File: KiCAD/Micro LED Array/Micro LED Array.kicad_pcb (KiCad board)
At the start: 2 copper layers, 8 x 32 mm, 57 parts, among them J1 JST-XH

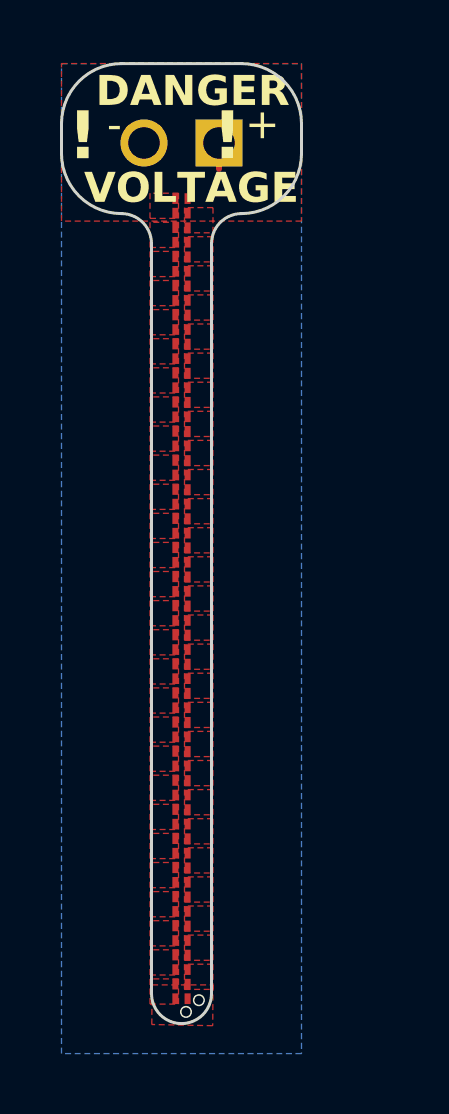
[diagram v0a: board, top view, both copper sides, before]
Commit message: Current setup
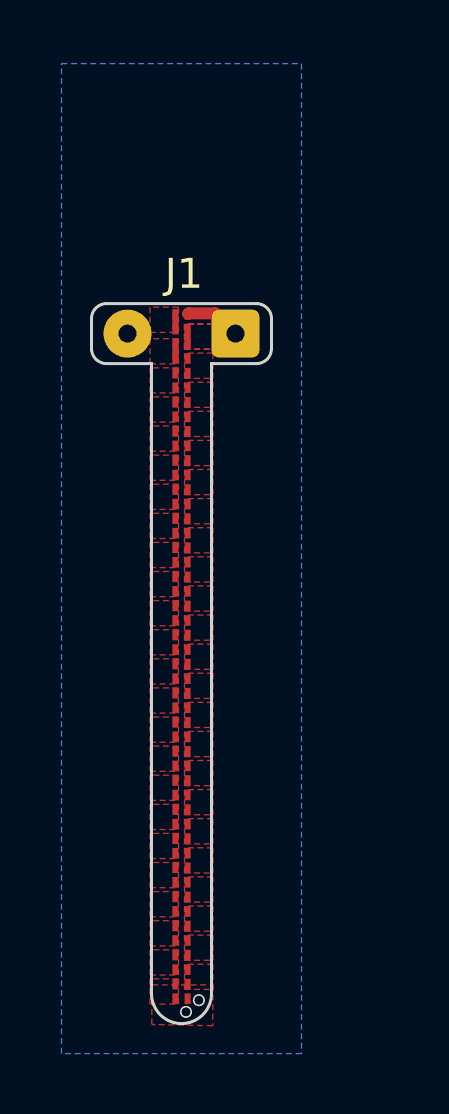
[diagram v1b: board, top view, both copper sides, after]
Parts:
- removed D13, D14, D15, D16, D5, D6, D7, D8: LED, Custom footprints:LED_APG0603SEC-E-TT_KNB
- J1: footprint Custom footprints:JST_B2B-XH-A -> Connector_Wire:SolderWire-0.1sqmm_1x02_P3.6mm_D0.4mm_OD1mm; moved to F.Cu
- moved J1 6.10 mm to (38.3, 25.5), turned to 180 degrees
- moved D1 5.33 mm to (36.5, 26.3), turned to -90 degrees
- moved D2 4.36 mm to (36.5, 25.8), turned to 90 degrees
- moved D3 3.38 mm to (36.5, 25.4), turned to -90 degrees
- moved D4 2.41 mm to (36.5, 24.9), turned to 90 degrees
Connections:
- D1 pad 2: VDD -> Net-(D1-A)
- D12 pad 2: Net-(D12-A) -> Net-(D1-K)
- D2 pad 1: Net-(D2-K) -> Net-(D1-A)
- D2 pad 2: Net-(D1-K) -> Net-(D2-A)
- D3 pad 1: Net-(D3-K) -> Net-(D2-A)
- D3 pad 2: Net-(D2-K) -> Net-(D3-A)
- D4 pad 1: Net-(D4-K) -> Net-(D3-A)
- D4 pad 2: Net-(D3-K) -> VDD
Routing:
- net VDD: track 0.87 -> 1.95 mm
- added copper zone on F.Cu, net Net-(D1-A)
- added copper zone on F.Cu, net Net-(D2-A)
- added copper zone on F.Cu, net Net-(D3-A)
- removed copper zone on F.Cu, net Net-(D12-A)
- removed copper zone on F.Cu, net Net-(D13-A)
- removed copper zone on F.Cu, net Net-(D14-A)
- removed copper zone on F.Cu, net Net-(D15-A)
- removed copper zone on F.Cu, net Net-(D16-A)
- removed copper zone on F.Cu, net Net-(D2-K)
- removed copper zone on F.Cu, net Net-(D3-K)
- removed copper zone on F.Cu, net Net-(D4-K)
- removed copper zone on F.Cu, net Net-(D5-K)
- removed copper zone on F.Cu, net Net-(D6-K)
- removed copper zone on F.Cu, net Net-(D7-K)
- removed copper zone on F.Cu, net VDD
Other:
- board size 8 x 32 mm -> 6 x 24 mm
- board text removed: "! !"
- board text removed: "+"
- board text removed: "-"
- board text removed: "DANGER"
- board text removed: "VOLTAGE"

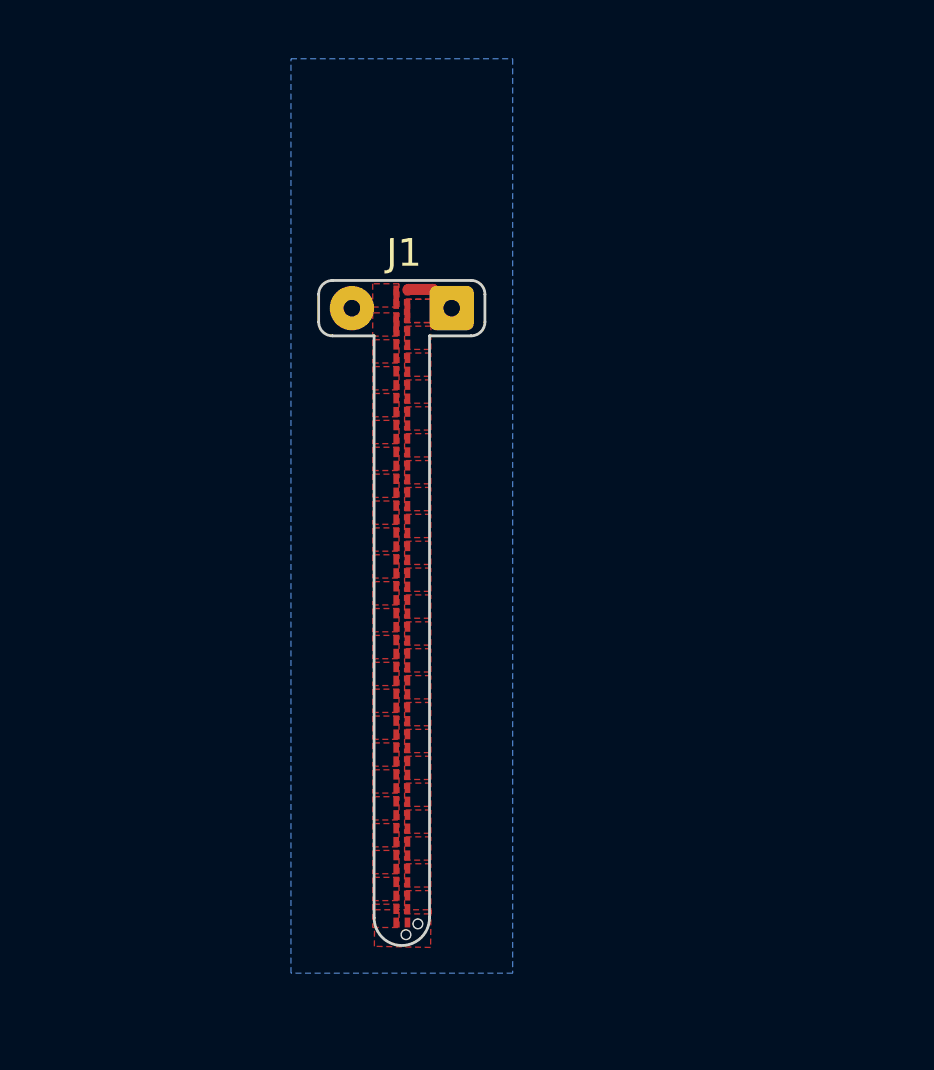
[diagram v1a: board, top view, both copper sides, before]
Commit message: Initial draft
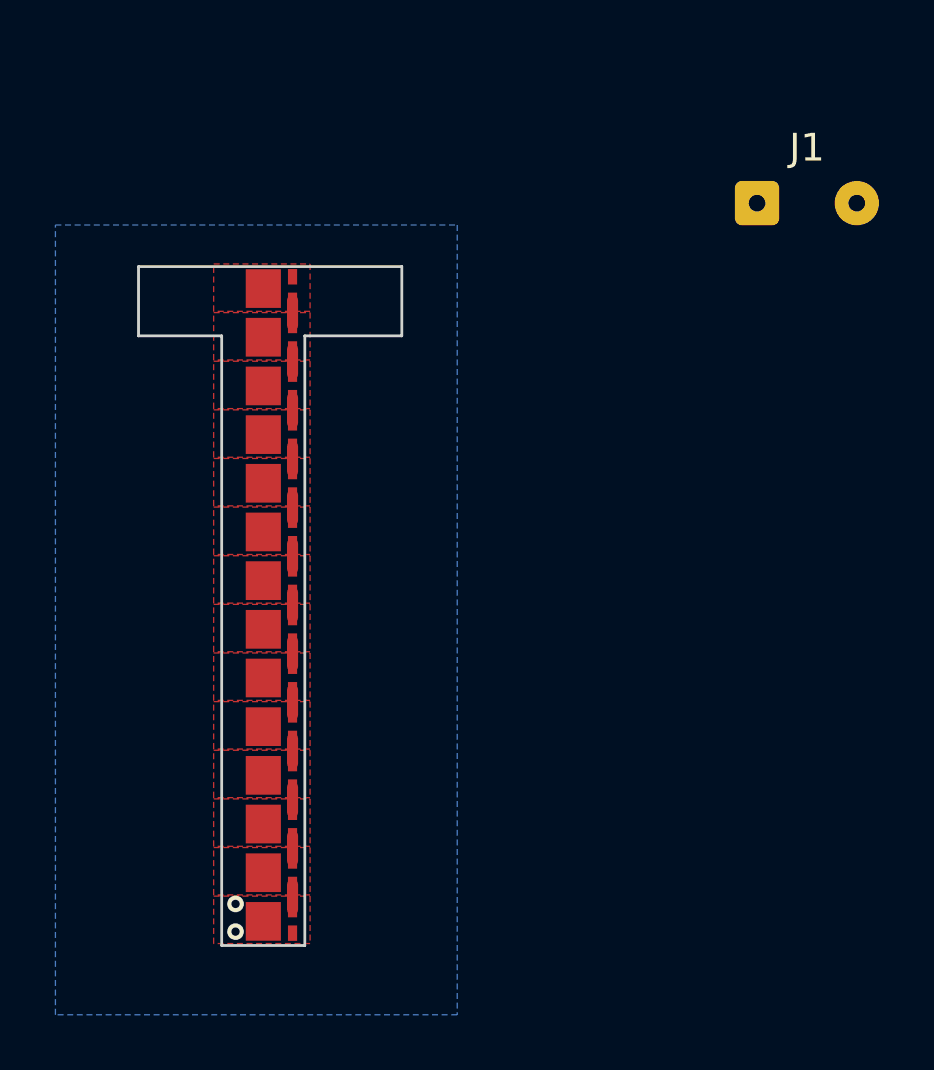
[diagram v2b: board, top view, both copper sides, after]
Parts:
- removed D17, D18, D19, D20, D21, D22, D23, D24, D25, D26, D27, D28, D29, D30, D31, D32, D33, D34, D35, D36, D37, D38, D39, D40, D41, D42, D43, D44, D45, D46, D47, D48, D49, D50, D51, D52, D53, D54, D55, D56: LED, Custom footprints:LED_APG0603SEC-E-TT_KNB
- added D13: LED, Custom footprints:LED_XLAMP_XE-G_CRW, F.Cu at (31.8, 45.9)
- added D14: LED, Custom footprints:LED_XLAMP_XE-G_CRW, F.Cu at (31.8, 47.6)
- added D5: LED, Custom footprints:LED_XLAMP_XE-G_CRW, F.Cu at (31.8, 31.8)
- added D6: LED, Custom footprints:LED_XLAMP_XE-G_CRW, F.Cu at (31.8, 33.6)
- added D7: LED, Custom footprints:LED_XLAMP_XE-G_CRW, F.Cu at (31.8, 35.3)
- added D8: LED, Custom footprints:LED_XLAMP_XE-G_CRW, F.Cu at (31.8, 37.1)
- D1, D10, D11, D12, D2, D3, D4, D9: footprint Custom footprints:LED_APG0603SEC-E-TT_KNB -> Custom footprints:LED_XLAMP_XE-G_CRW
- moved D12 17.9 mm to (31.8, 44.1), turned to 180 degrees
- moved D11 15.8 mm to (31.8, 42.4), turned to 180 degrees
- moved D10 13.7 mm to (31.8, 40.6), turned to 180 degrees
- moved J1 11.7 mm to (49.3, 21.7), turned to 0 degrees
- moved D9 11.6 mm to (31.8, 38.8), turned to 180 degrees
- moved D4 7.02 mm to (31.8, 30.1), turned to 180 degrees
- moved D3 5.56 mm to (31.8, 28.3), turned to 180 degrees
- moved D1 4.95 mm to (31.8, 24.8), turned to 180 degrees
- moved D2 4.76 mm to (31.8, 26.6), turned to 180 degrees
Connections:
- D1 pad 2: Net-(D1-A) -> VDD
- D11 pad 1: Net-(D10-A) -> Net-(D11-K)
- D11 pad 2: Net-(D11-A) -> Net-(D10-K)
- D12 pad 1: Net-(D11-A) -> Net-(D12-K)
- D12 pad 2: Net-(D1-K) -> Net-(D11-K)
- D2 pad 1: Net-(D1-A) -> Net-(D2-K)
- D2 pad 2: Net-(D2-A) -> Net-(D1-K)
- D3 pad 1: Net-(D2-A) -> Net-(D3-K)
- D3 pad 2: Net-(D3-A) -> Net-(D2-K)
- D4 pad 1: Net-(D3-A) -> Net-(D4-K)
- D4 pad 2: VDD -> Net-(D3-K)
- D9 pad 1: Net-(D17-A) -> Net-(D10-A)
- D9 pad 2: Net-(D10-K) -> Net-(D8-K)
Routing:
- net VDD: track 1.95 -> 0.00 mm
- net Net-(D8-K): track 0.00 -> 0.91 mm
- net Net-(D7-K): track 0.00 -> 0.91 mm
- net Net-(D6-K): track 0.00 -> 0.91 mm
- net Net-(D5-K): track 0.00 -> 0.91 mm
- net Net-(D2-K): track 0.00 -> 0.91 mm
- net Net-(D13-K): track 0.00 -> 0.91 mm
- net Net-(D12-K): track 0.00 -> 0.91 mm
- net Net-(D11-K): track 0.00 -> 0.91 mm
- net Net-(D10-A): track 0.00 -> 0.91 mm
- net Net-(D1-K): track 0.00 -> 0.91 mm
- net Net-(D4-K): track 0.00 -> 0.91 mm
- net Net-(D3-K): track 0.00 -> 0.91 mm
- net Net-(D10-K): track 0.00 -> 0.91 mm
- added copper zone on F.Cu, net Net-(D11-K)
- added copper zone on F.Cu, net Net-(D12-K)
- added copper zone on F.Cu, net Net-(D13-K)
- added copper zone on F.Cu, net Net-(D2-K)
- added copper zone on F.Cu, net Net-(D3-K)
- added copper zone on F.Cu, net Net-(D4-K)
- added copper zone on F.Cu, net Net-(D5-K)
- added copper zone on F.Cu, net Net-(D6-K)
- added copper zone on F.Cu, net Net-(D7-K)
- added copper zone on F.Cu, net Net-(D8-K)
- removed copper zone on F.Cu, net Net-(D1-A)
- removed copper zone on F.Cu, net Net-(D11-A)
- removed copper zone on F.Cu, net Net-(D17-A)
- removed copper zone on F.Cu, net Net-(D17-K)
- removed copper zone on F.Cu, net Net-(D18-K)
- removed copper zone on F.Cu, net Net-(D19-K)
- removed copper zone on F.Cu, net Net-(D2-A)
- removed copper zone on F.Cu, net Net-(D20-K)
- removed copper zone on F.Cu, net Net-(D21-K)
- removed copper zone on F.Cu, net Net-(D22-K)
- removed copper zone on F.Cu, net Net-(D23-K)
- removed copper zone on F.Cu, net Net-(D24-K)
- removed copper zone on F.Cu, net Net-(D25-A)
- removed copper zone on F.Cu, net Net-(D25-K)
- removed copper zone on F.Cu, net Net-(D26-A)
- removed copper zone on F.Cu, net Net-(D27-A)
- removed copper zone on F.Cu, net Net-(D28-A)
- removed copper zone on F.Cu, net Net-(D29-A)
- removed copper zone on F.Cu, net Net-(D3-A)
- removed copper zone on F.Cu, net Net-(D30-A)
- removed copper zone on F.Cu, net Net-(D31-A)
- removed copper zone on F.Cu, net Net-(D33-K)
- removed copper zone on F.Cu, net Net-(D34-K)
- removed copper zone on F.Cu, net Net-(D35-K)
- removed copper zone on F.Cu, net Net-(D36-K)
- removed copper zone on F.Cu, net Net-(D37-K)
- removed copper zone on F.Cu, net Net-(D38-K)
- removed copper zone on F.Cu, net Net-(D39-K)
- removed copper zone on F.Cu, net Net-(D40-K)
- removed copper zone on F.Cu, net Net-(D41-A)
- removed copper zone on F.Cu, net Net-(D41-K)
- removed copper zone on F.Cu, net Net-(D42-A)
- removed copper zone on F.Cu, net Net-(D43-A)
- removed copper zone on F.Cu, net Net-(D44-A)
- removed copper zone on F.Cu, net Net-(D45-A)
- removed copper zone on F.Cu, net Net-(D46-A)
- removed copper zone on F.Cu, net Net-(D47-A)
- removed copper zone on F.Cu, net Net-(D49-K)
- removed copper zone on F.Cu, net Net-(D50-K)
- removed copper zone on F.Cu, net Net-(D51-K)
- removed copper zone on F.Cu, net Net-(D52-K)
- removed copper zone on F.Cu, net Net-(D53-K)
- removed copper zone on F.Cu, net Net-(D54-K)
- removed copper zone on F.Cu, net Net-(D55-K)
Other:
- board size 6 x 24 mm -> 9.5 x 24.5 mm
- board text removed: "HIGH VOLTAGE! 20 mA Max"
